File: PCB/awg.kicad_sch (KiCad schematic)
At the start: 62 parts, among them J1 02x05, J2 02x02, J3 01x02, J4 01x02, U1 LM2904, U2 LM2904, U3 LM2904, U4 DG403, U5 r1283

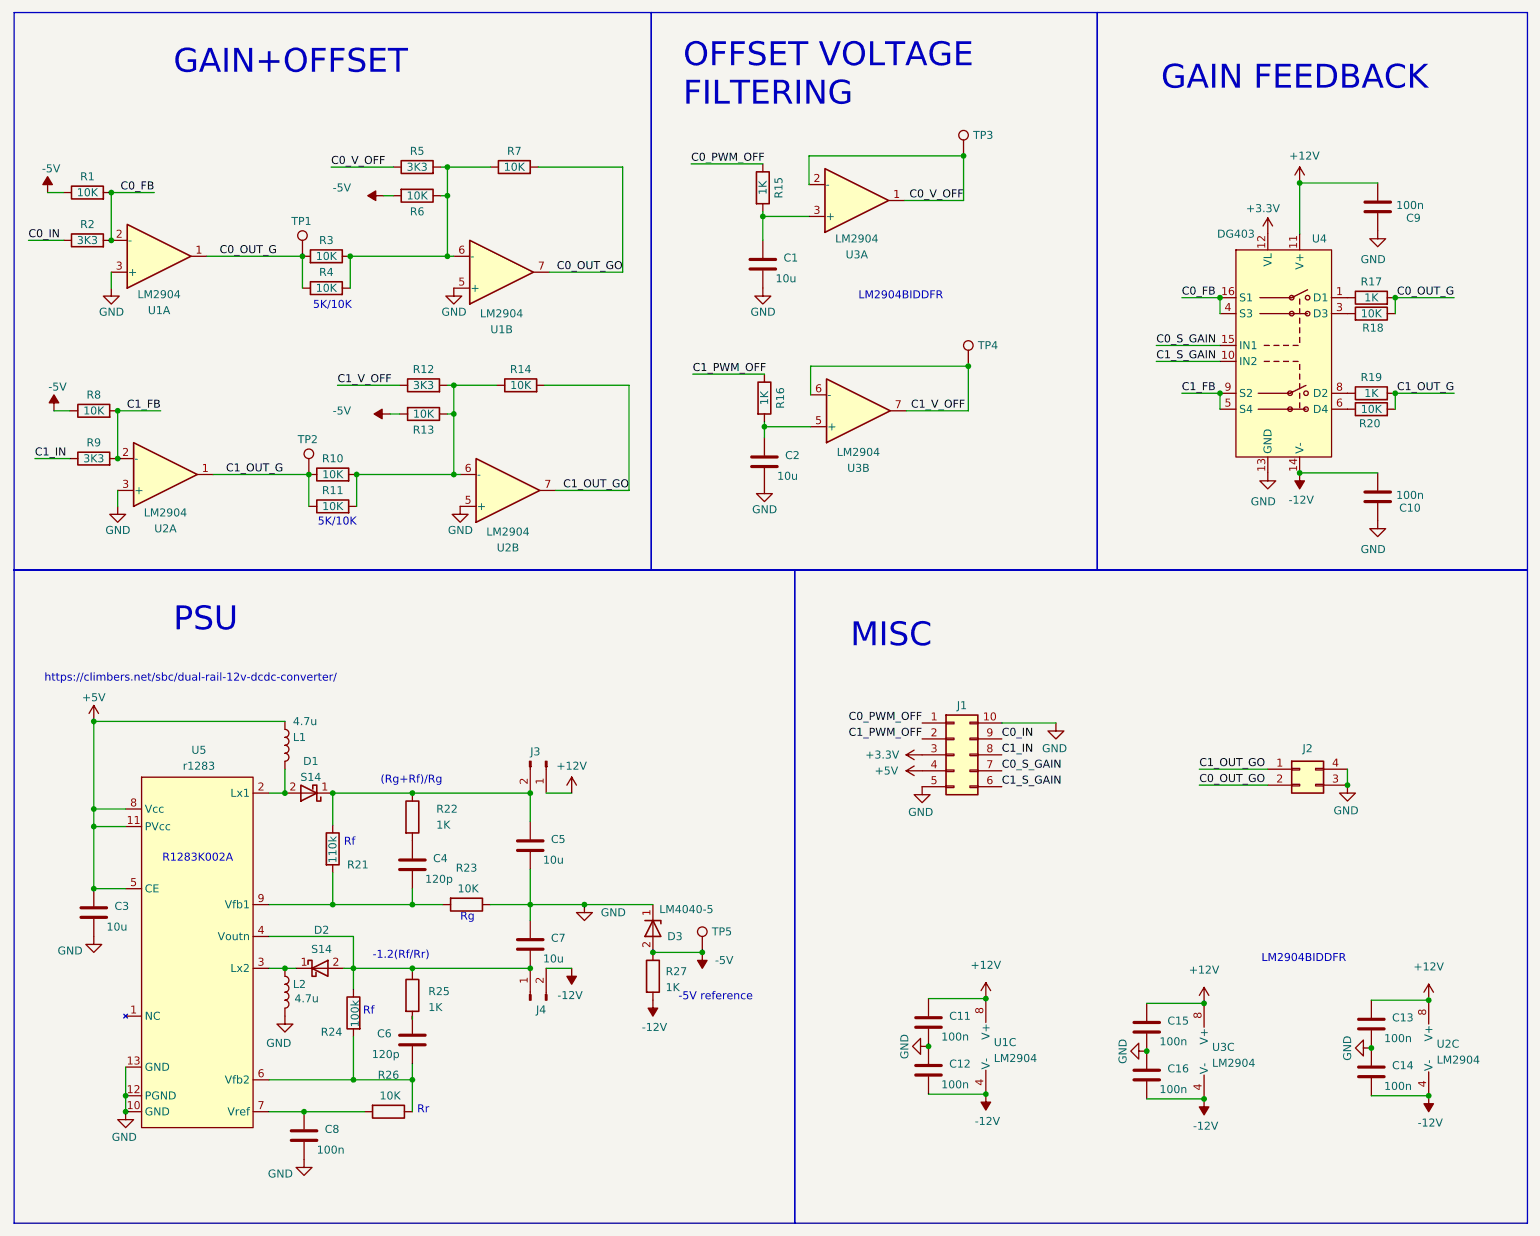
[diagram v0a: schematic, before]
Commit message: 9/14/23
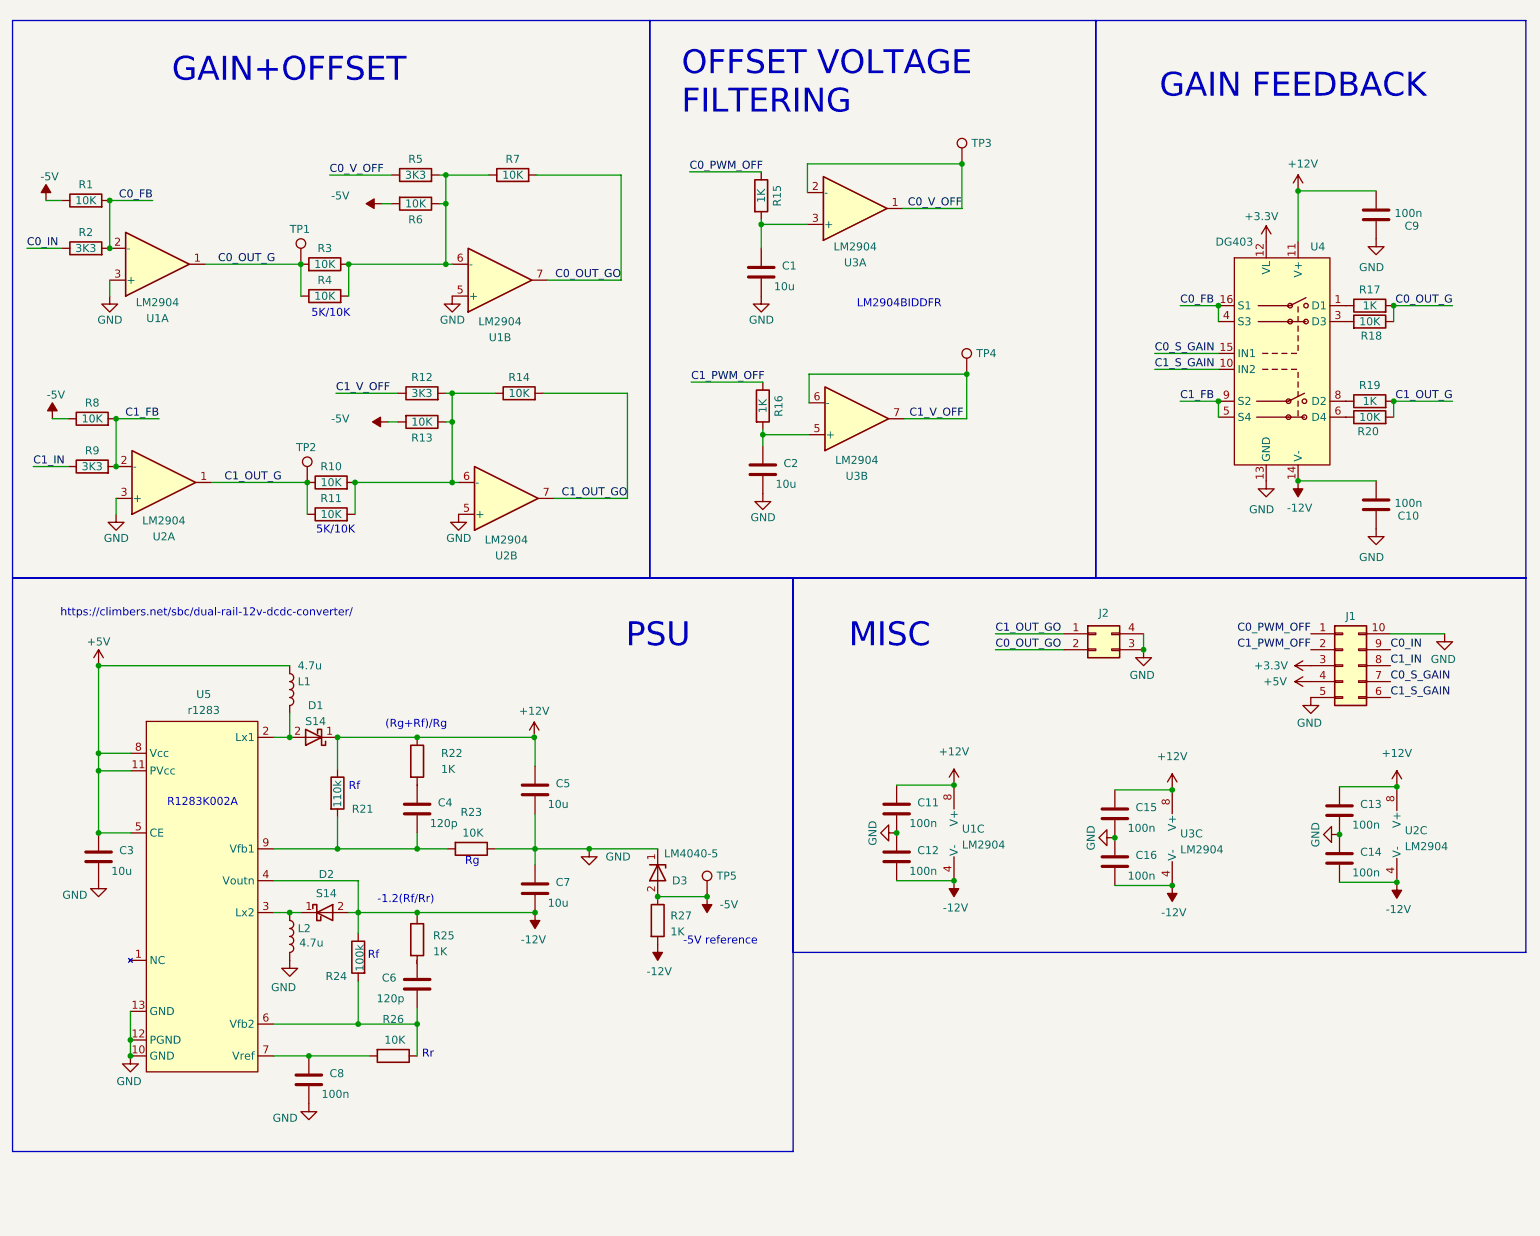
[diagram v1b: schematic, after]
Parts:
- removed J3, J4: 01x02, Connector_PinHeader_2.54mm:PinHeader_1x02_P2.54mm_Vertical, symbol Connector:Conn_01x02_Pin
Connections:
- net +12V: now also C5.1, D1.1 (K), R21.1, R22.1
- net -12V: now also C7.2, D2.2 (A), R24.1, R25.1, U5.4 (Voutn)
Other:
- moved on the sheet: C1, C10, C11, C12, C13, C14, C15, C16, C2, C3, C4, C5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
